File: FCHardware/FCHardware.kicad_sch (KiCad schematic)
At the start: 18 parts, among them U1 ESC_Xrotor_65A_4in1, U4 TPS629203, U5 MPU-6050

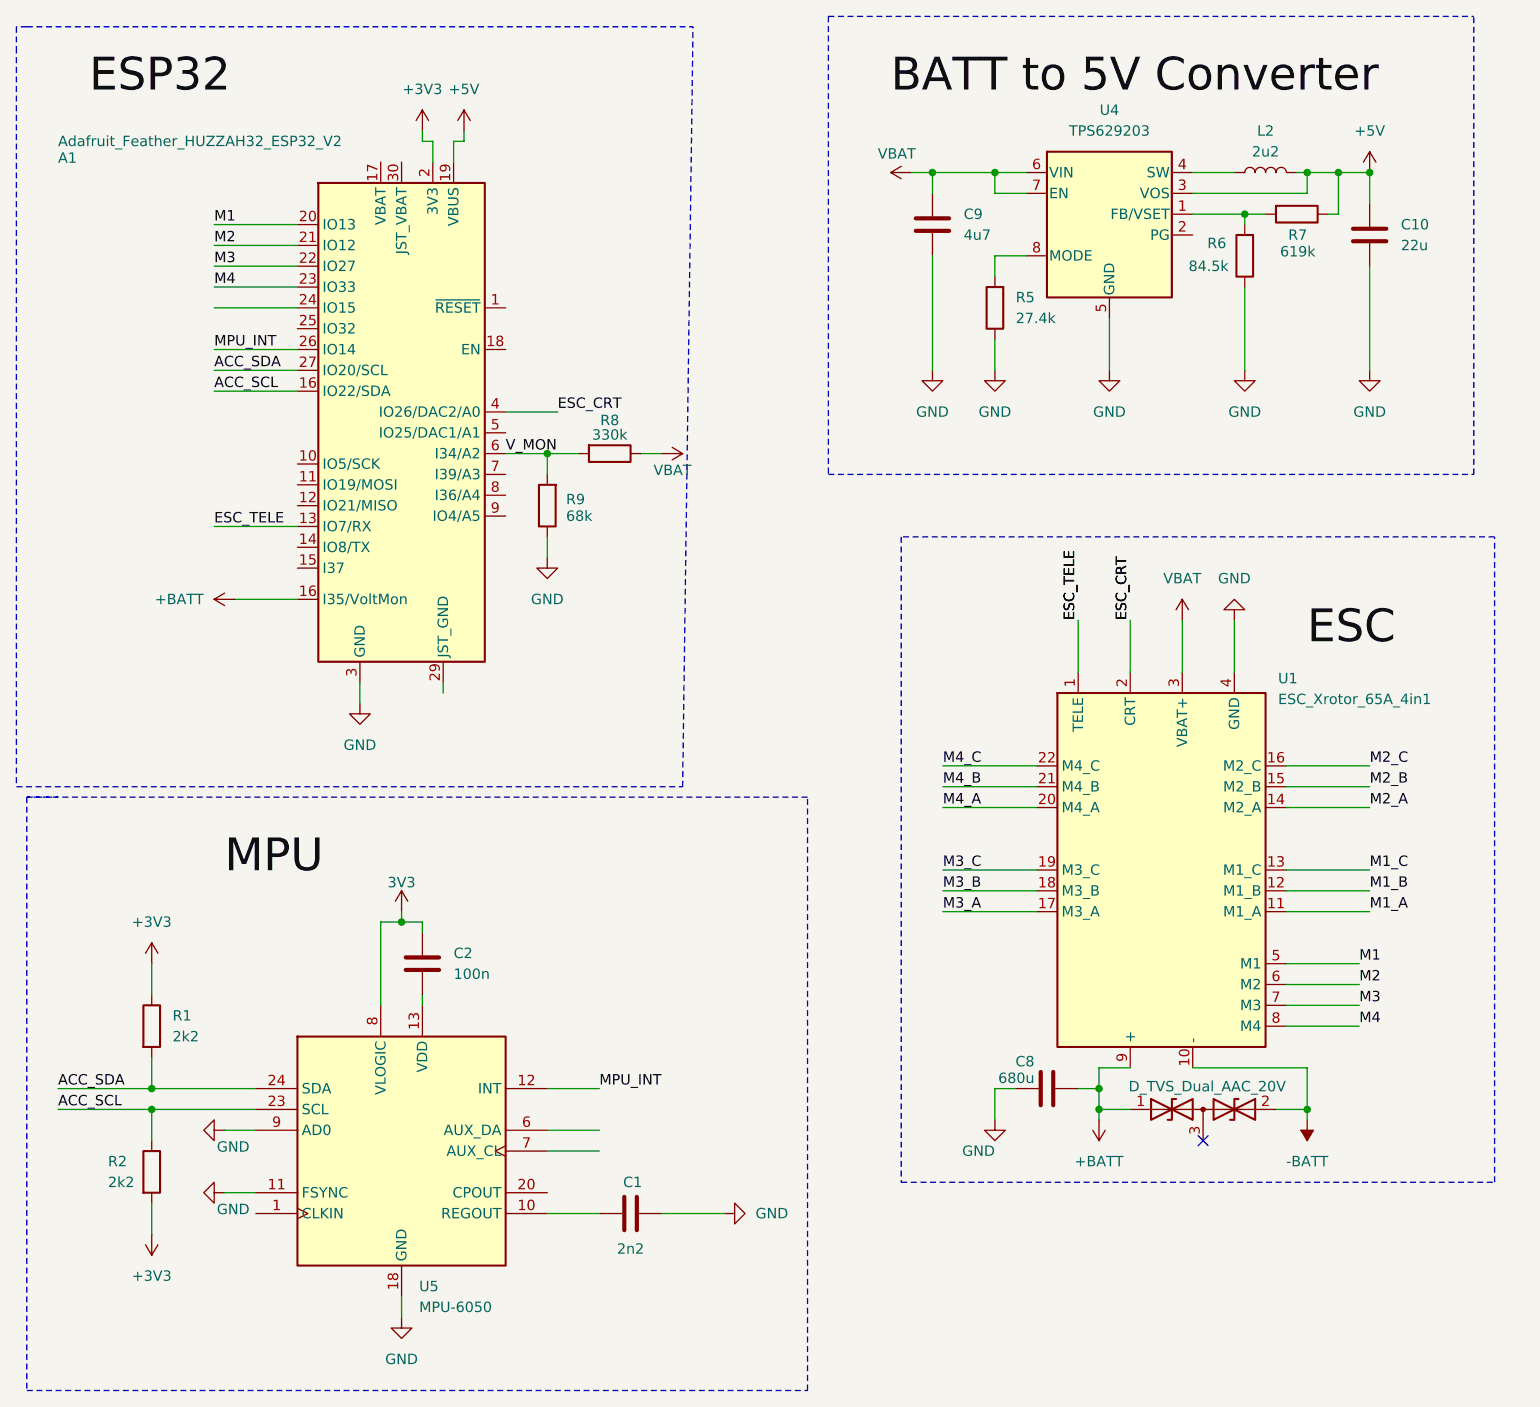
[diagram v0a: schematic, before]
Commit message: Updated documentation
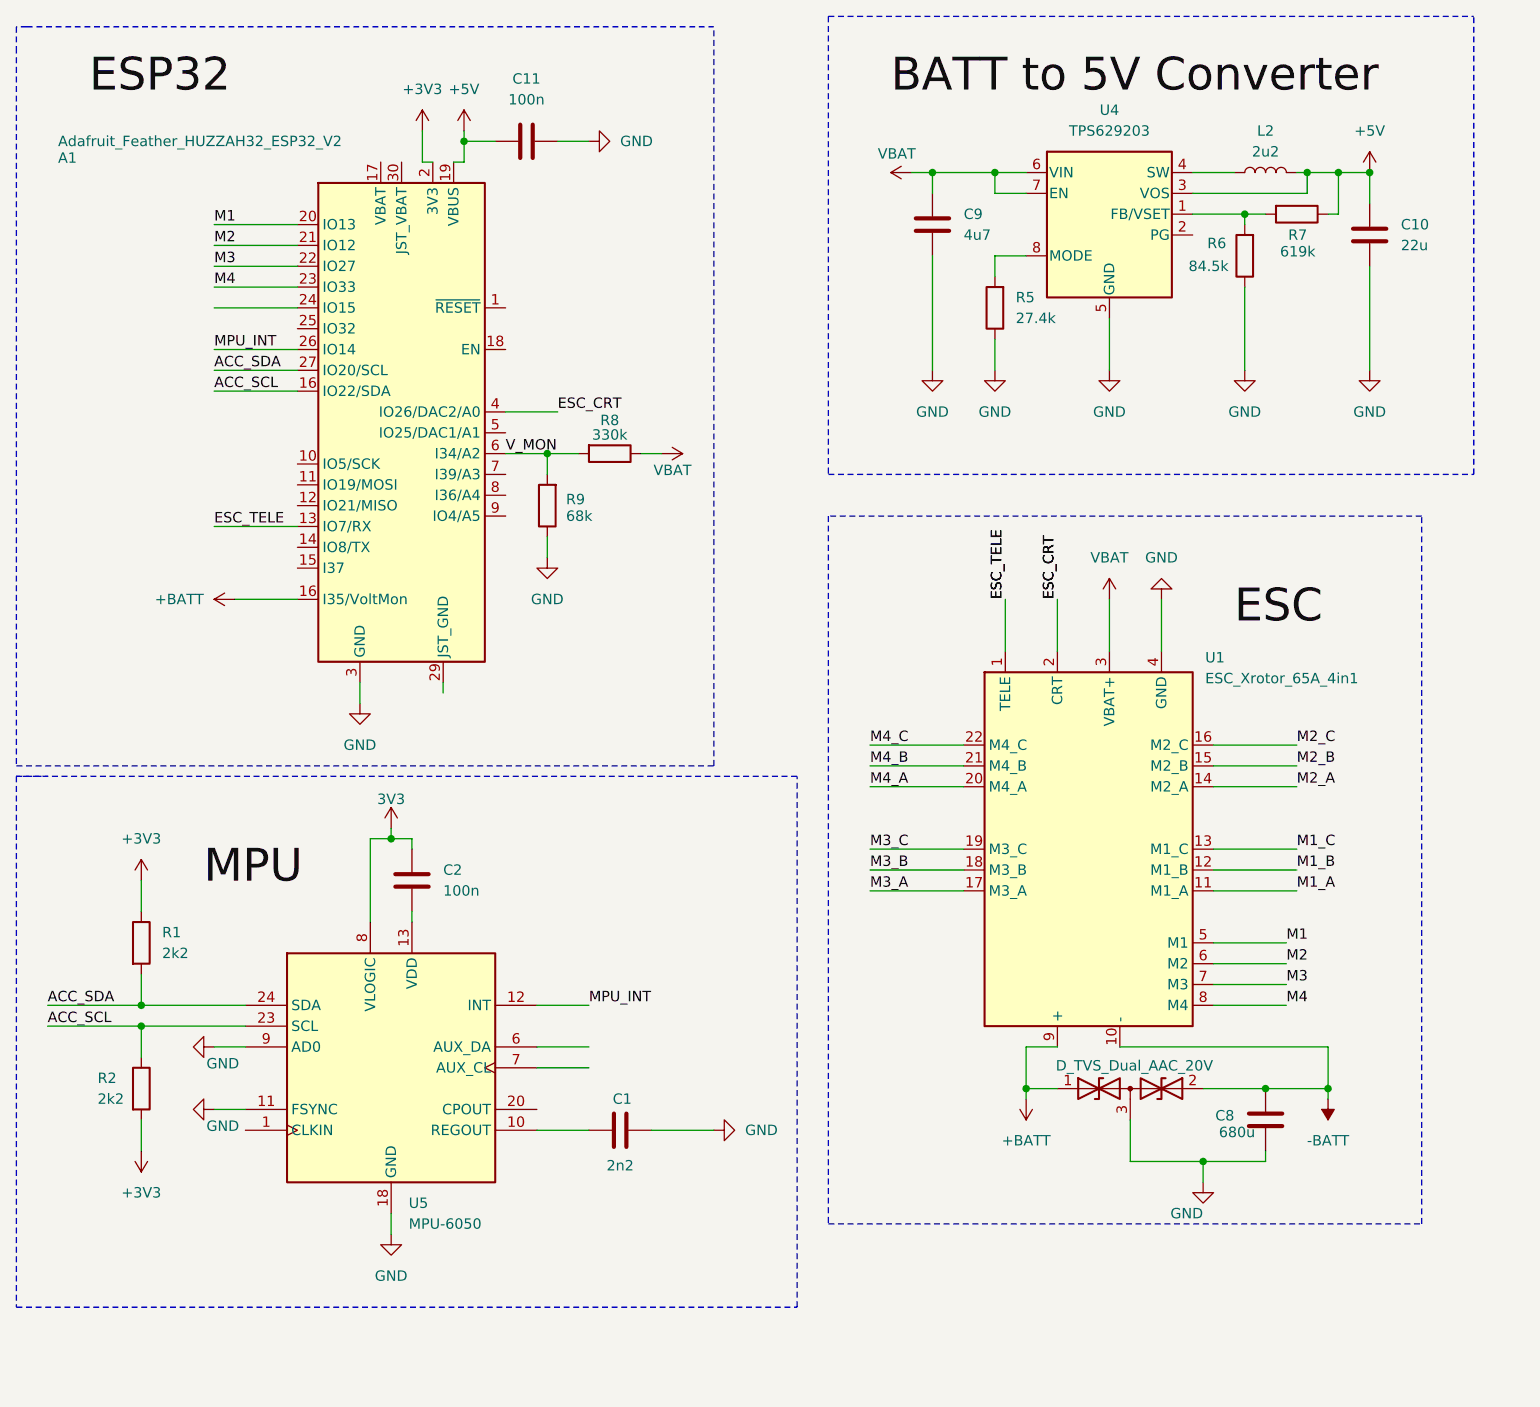
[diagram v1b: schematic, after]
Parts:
- added C11: 100n, symbol Device:C
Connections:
- net +5V: now also C11.1
- net +BATT: no longer C8.2
- net -BATT: now also C8.2
- net GND: now also D1.3 (common), C11.2
- no-connect marks 1 -> 0
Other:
- moved on the sheet: C1, C2, C8, R1, R2, U1, U5
